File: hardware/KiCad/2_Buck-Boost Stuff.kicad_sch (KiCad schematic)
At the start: 51 parts, among them Q3 BSC030N08NS5, Q5 BSC030N08NS5, Q6 BSC030N08NS5, Q7 BSC030N08NS5, U2 CC6937S8-3FB020, U3 CC6937S8-3FB020

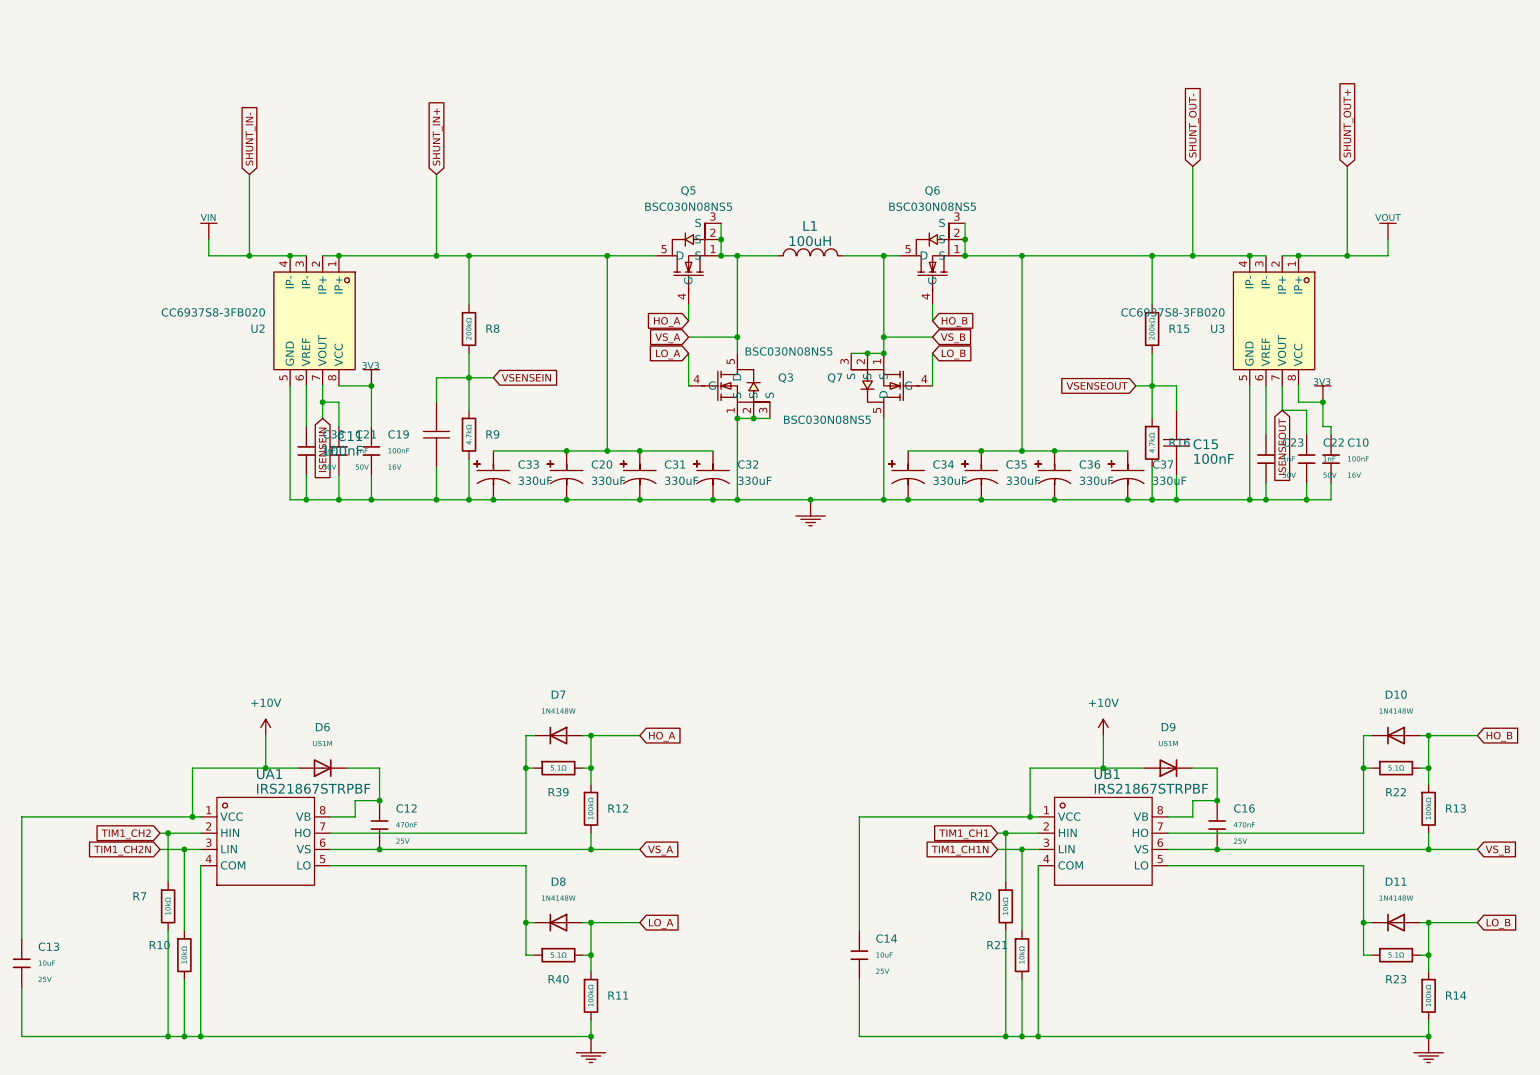
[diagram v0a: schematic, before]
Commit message: updates
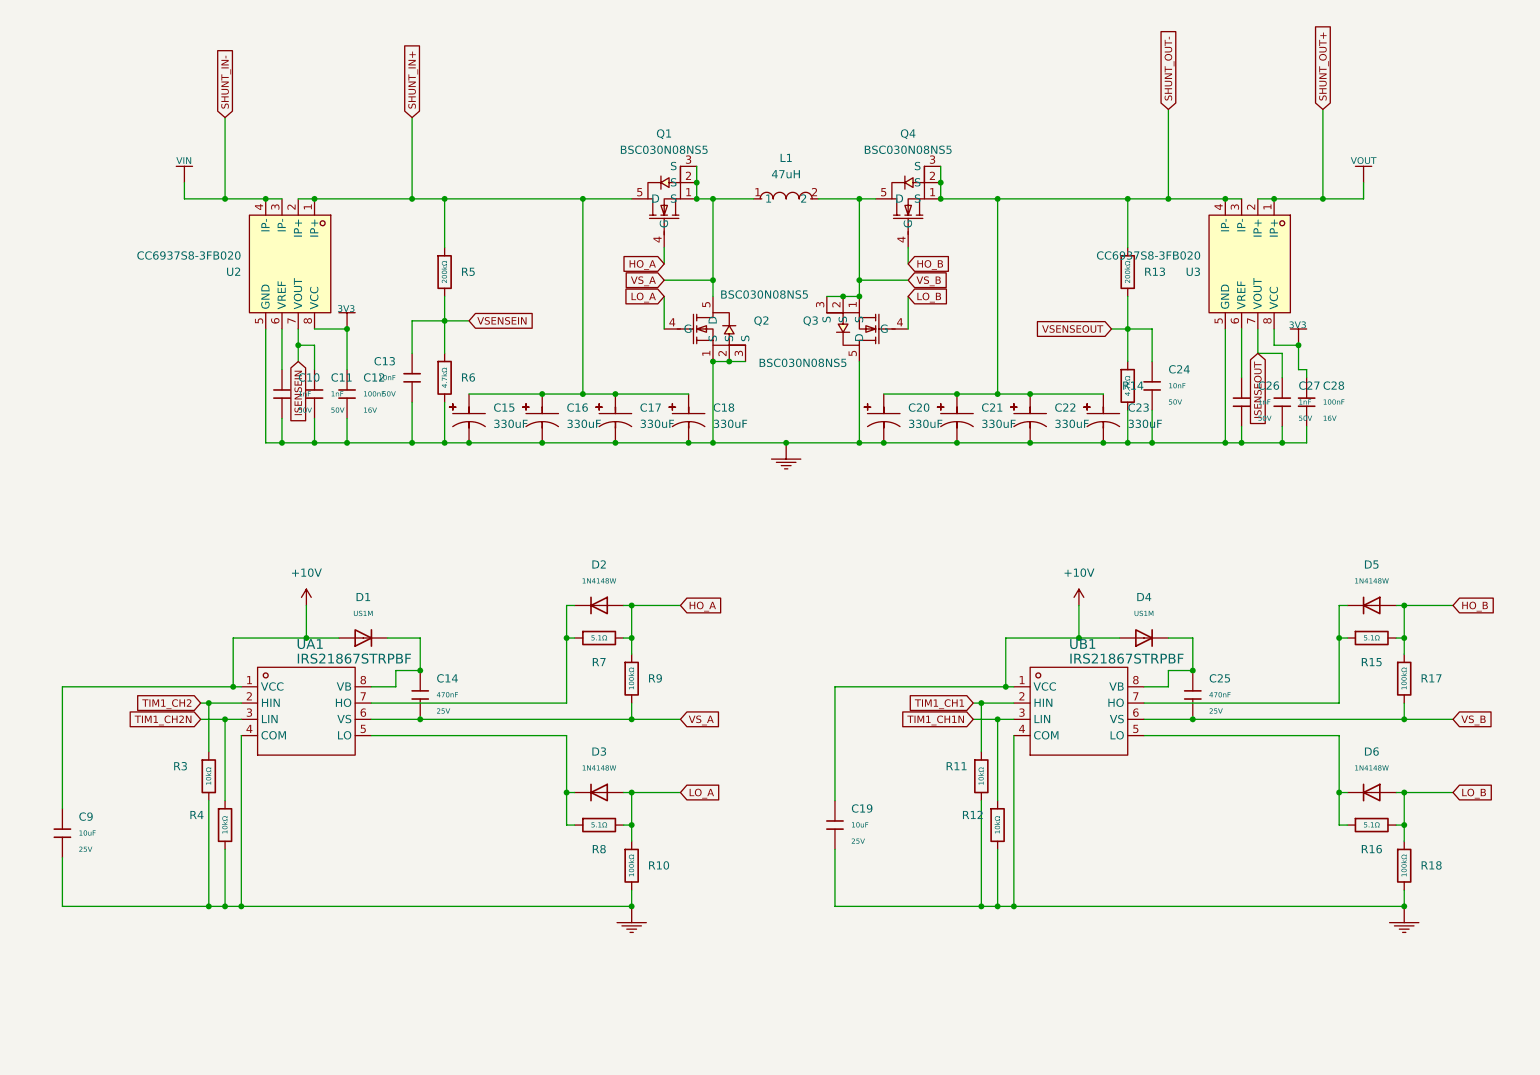
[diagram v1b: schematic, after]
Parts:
- removed C11, C15: 100nF, ProPrj_STM-easyedapro:C0603, symbol ProPrj_STM-easyedapro:100nF
- removed L1: 100uH, ProPrj_STM-easyedapro:IND-SMD_L6.0-W6.0, symbol ProPrj_STM-easyedapro:100uH
- added C13, C24: 10nF, PCM_JLCPCB:C_0402, symbol JLCPCB-Capacitors:0402,10nF
- added L1: 47uH, easyeda2kicad:IND-TH_L32.2-W22.2_CPEX3222L, symbol easyeda2kicad:CPEX3222L-470MC-RS
- renumbered C38 to C10, C21 to C11, C19 to C12, C12 to C14, C33 to C15, C20 to C16, C31 to C17, C32 to C18, C14 to C19, C34 to C20, C35 to C21, C36 to C22, C37 to C23, C16 to C25, C23 to C26, C22 to C27, C10 to C28, C13 to C9, D6 to D1, D7 to D2, D8 to D3, D9 to D4, D10 to D5, D11 to D6, Q5 to Q1, Q3 to Q2, Q7 to Q3, Q6 to Q4, R11 to R10, R20 to R11, R21 to R12, R15 to R13, R16 to R14, R22 to R15, R23 to R16, R13 to R17, R14 to R18, R7 to R3, R10 to R4, R8 to R5, R9 to R6, R39 to R7, R40 to R8, R12 to R9
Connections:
- net GND: now also C13.2, C24.2
- net VSENSEIN: now also C13.1
- net VSENSEOUT: now also C24.1
- net VS_A: now also L1.1
- net VS_B: now also L1.2
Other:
- moved on the sheet: C10, C11, C12, C14, C15, C16, C17, C18, C19, C20, C21, C22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
